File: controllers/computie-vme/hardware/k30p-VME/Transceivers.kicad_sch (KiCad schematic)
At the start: 5 parts, among them U10 74ABT16245DL, U11 74ABT16245DL, U12 74ABT16245DL, U14 74ABT16245DL, U16 74ABT16245DL

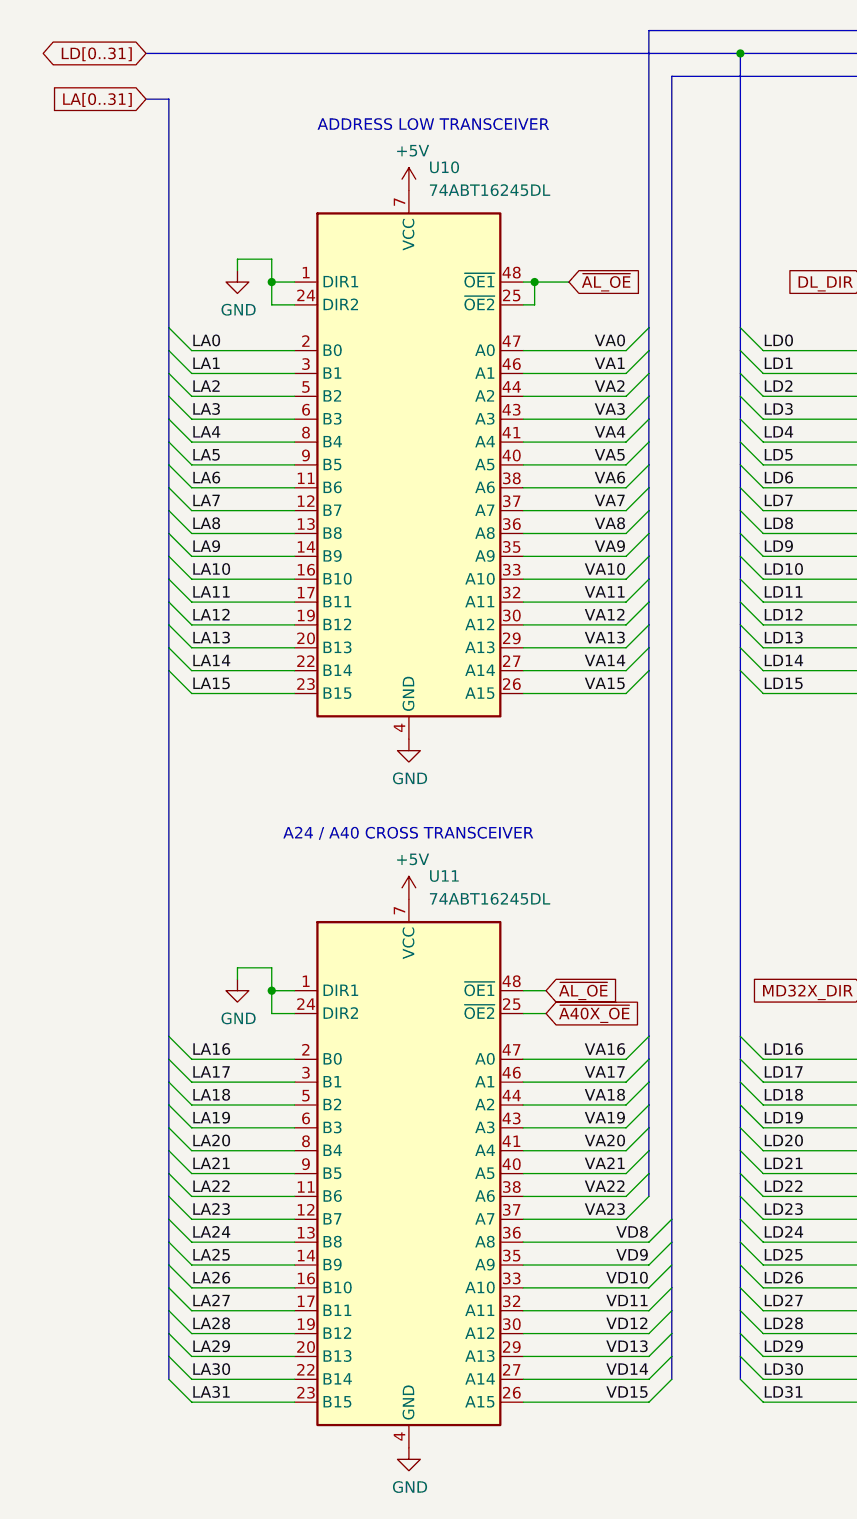
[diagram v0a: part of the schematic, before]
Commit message: WIP on k30p-VME
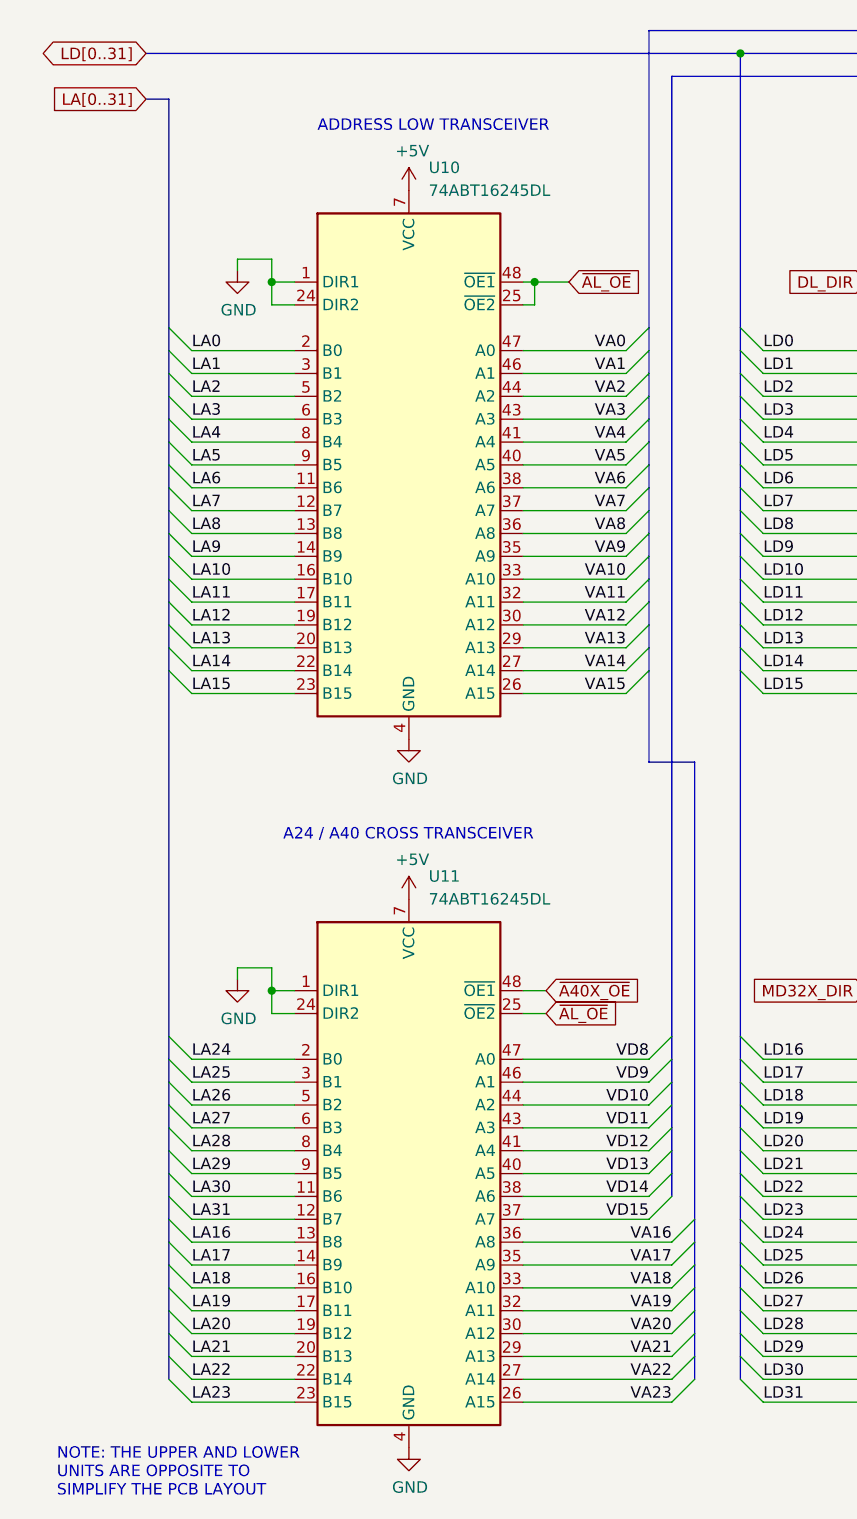
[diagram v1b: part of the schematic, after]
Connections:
- net LA16: now also U11.13 (B8); no longer U11.2 (B0)
- net LA17: now also U11.14 (B9); no longer U11.3 (B1)
- net LA18: now also U11.16 (B10); no longer U11.5 (B2)
- net LA19: now also U11.17 (B11); no longer U11.6 (B3)
- net LA20: now also U11.19 (B12); no longer U11.8 (B4)
- net LA21: now also U11.20 (B13); no longer U11.9 (B5)
- net LA22: now also U11.22 (B14); no longer U11.11 (B6)
- net LA23: now also U11.23 (B15); no longer U11.12 (B7)
- net LA24: now also U11.2 (B0); no longer U11.13 (B8)
- net LA25: now also U11.3 (B1); no longer U11.14 (B9)
- net LA26: now also U11.5 (B2); no longer U11.16 (B10)
- net LA27: now also U11.6 (B3); no longer U11.17 (B11)
- net LA28: now also U11.8 (B4); no longer U11.19 (B12)
- net LA29: now also U11.9 (B5); no longer U11.20 (B13)
- net LA30: now also U11.11 (B6); no longer U11.22 (B14)
- net LA31: now also U11.12 (B7); no longer U11.23 (B15)
- net VA16: now also U11.36 (A8); no longer U11.47 (A0)
- net VA17: now also U11.35 (A9); no longer U11.46 (A1)
- net VA18: now also U11.33 (A10); no longer U11.44 (A2)
- net VA19: now also U11.32 (A11); no longer U11.43 (A3)
- net VA20: now also U11.30 (A12); no longer U11.41 (A4)
- net VA21: now also U11.29 (A13); no longer U11.40 (A5)
- net VA22: now also U11.27 (A14); no longer U11.38 (A6)
- net VA23: now also U11.26 (A15); no longer U11.37 (A7)
- net VD10: now also U11.44 (A2); no longer U11.33 (A10)
- net VD11: now also U11.43 (A3); no longer U11.32 (A11)
- net VD12: now also U11.41 (A4); no longer U11.30 (A12)
- net VD13: now also U11.40 (A5); no longer U11.29 (A13)
- net VD14: now also U11.38 (A6); no longer U11.27 (A14)
- net VD15: now also U11.37 (A7); no longer U11.26 (A15)
- net VD8: now also U11.47 (A0); no longer U11.36 (A8)
- net VD9: now also U11.46 (A1); no longer U11.35 (A9)
- net ~{A40X_OE}: now also U11.48 (~{OE1}); no longer U11.25 (~{OE2})
- net ~{AL_OE}: now also U11.25 (~{OE2}); no longer U11.48 (~{OE1})
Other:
- note added: "NOTE: THE UPPER AND LOWER UNITS ARE OPPOSITE TO SIMPLIFY THE PCB LAYOUT"
